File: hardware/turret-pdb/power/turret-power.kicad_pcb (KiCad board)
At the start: 2 copper layers, 70 x 58 mm, 21 parts, among them J1 Battery in, J10 Vision 5V, J11 Servo bus 7.5V, J12 Stack link, J2 12V bench, J3 Arm switch, J4 Pusher, U3 MP1584 7.5V, U4 MP1584 6V, U5 MP1584 5V

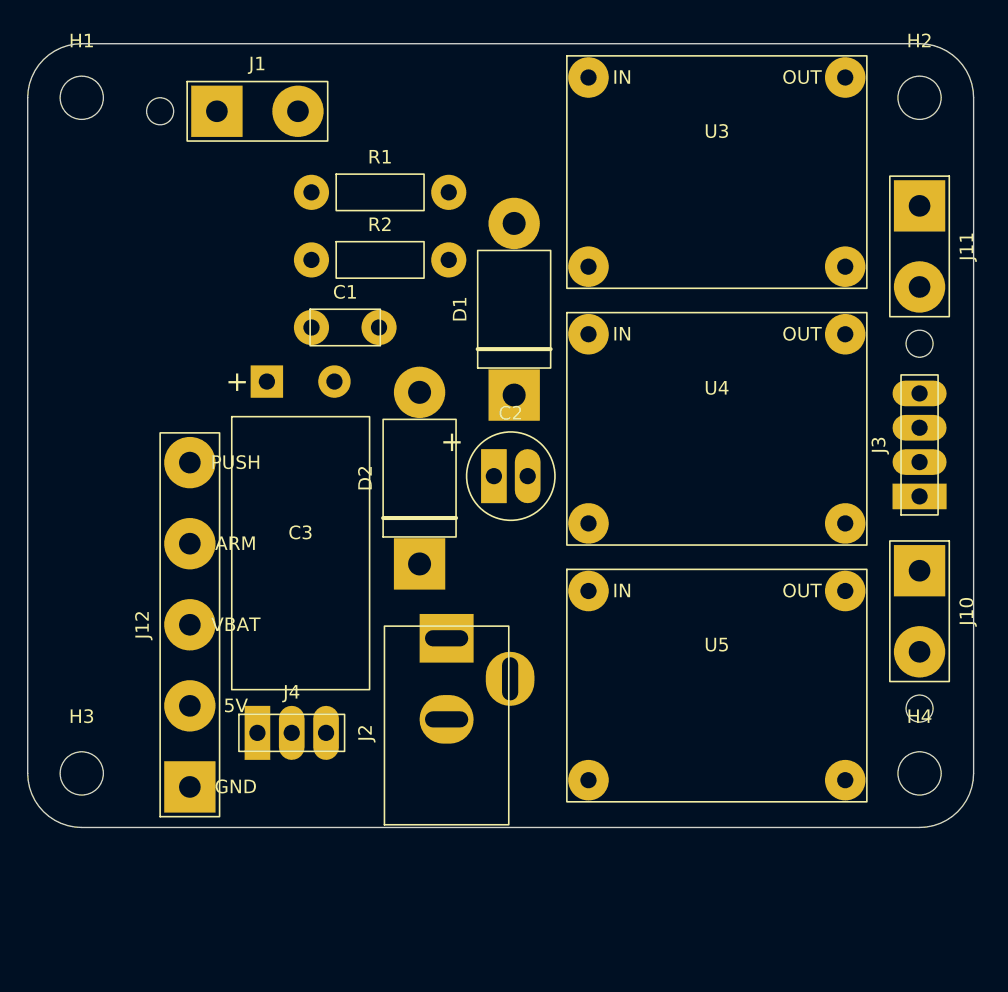
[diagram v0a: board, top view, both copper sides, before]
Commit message: Route the power board
Co-Authored-By: Claude Opus 5.5 <noreply@anthropic.com>
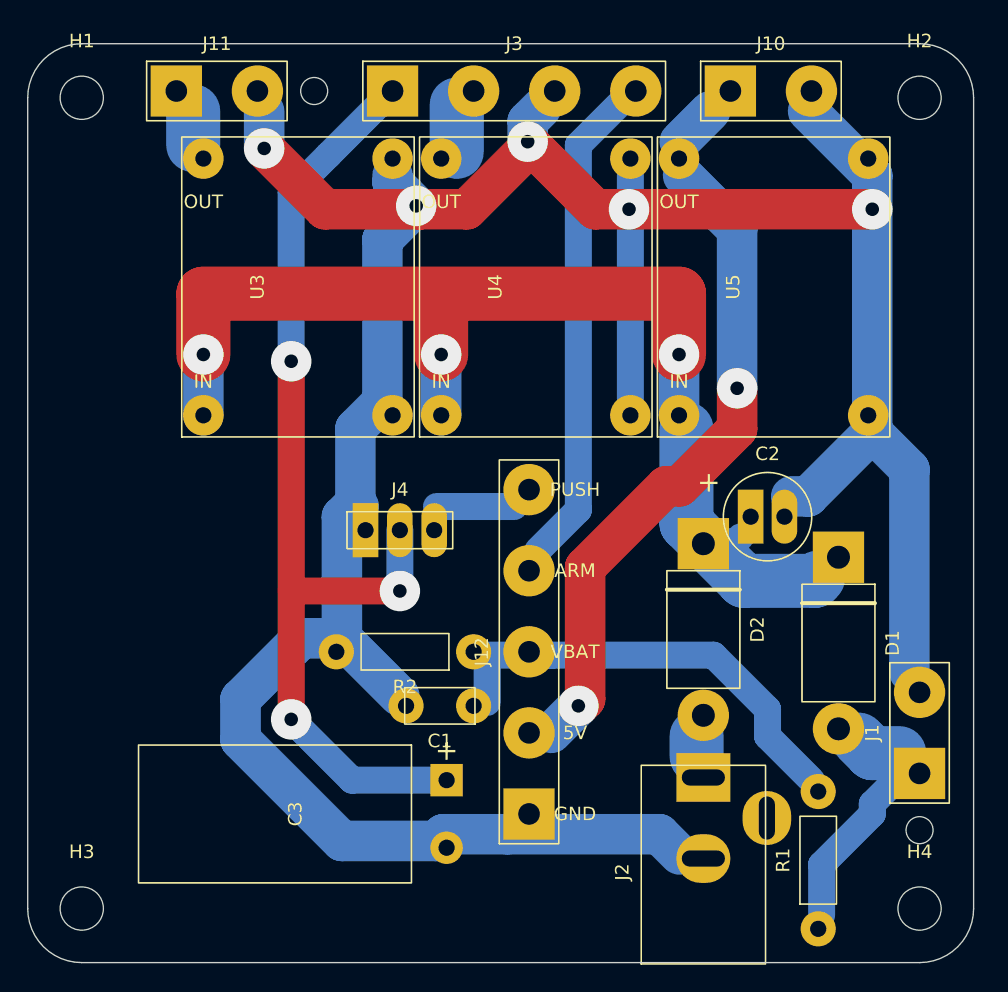
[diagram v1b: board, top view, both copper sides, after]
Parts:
- J10: footprint turret-power:WirePads_1x02_TieRight -> turret-power:WirePads_1x02_NoTie
- J3: footprint turret-power:PinHeader_1x04_P2.54mm -> turret-power:WirePads_1x04_NoTie
- moved J1 71.4 mm to (106.0, 94.0), turned to 90 degrees
- moved R1 66.2 mm to (98.5, 105.5), turned to 90 degrees
- moved J11 55.7 mm to (51.0, 43.5), turned to 0 degrees
- moved J3 49.2 mm to (67.0, 43.5), turned to 0 degrees
- moved J10 38.2 mm to (92.0, 43.5), turned to 0 degrees
- moved U3 37.9 mm to (53.0, 67.5), turned to 90 degrees
- moved C3 32.4 mm to (71.0, 94.5), turned to 270 degrees
- moved R2 31.4 mm to (73.0, 85.0), turned to 180 degrees
- moved C1 30.5 mm to (73.0, 89.0), turned to 180 degrees
- moved D1 26.8 mm to (100.0, 78.0), turned to 270 degrees
- moved J12 25.2 mm to (77.1, 97.0)
- moved J2 21.6 mm to (90.0, 94.3)
- moved D2 21.1 mm to (90.0, 77.0), turned to 270 degrees
- moved C2 19.2 mm to (93.5, 75.0)
- moved J4 17.0 mm to (65.0, 76.0)
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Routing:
- net GND: track 0.00 -> 218.7 mm, vias 0 -> 5
- net VIN: track 0.00 -> 82.9 mm, vias 0 -> 3
- net PUSH_6V: track 0.00 -> 75.5 mm, vias 0 -> 3
- net +5V: track 0.00 -> 52.4 mm, vias 0 -> 2
- net ARM_SENSE: track 0.00 -> 35.5 mm
- net VBAT_SENSE: track 0.00 -> 32.5 mm
- net VBAT: track 0.00 -> 16.0 mm
- net PUSH_SIG: track 0.00 -> 5.75 mm
- net +6V: track 0.00 -> 3.50 mm
- net +7V5: track 0.00 -> 2.50 mm
- net VJACK: track 0.00 -> 1.50 mm
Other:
- board size 70 x 58 mm -> 70 x 68 mm
